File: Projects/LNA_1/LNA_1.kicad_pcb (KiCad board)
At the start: 2 copper layers, 59.7 x 36.6 mm, 31 parts, among them J1 SMA-J-P-H-ST-EM1, J2 SMA-J-P-H-ST-EM1, J3 Barrel_Jack_MountingPin, Q1 Q_NPN_BEC, U1 BFU790F

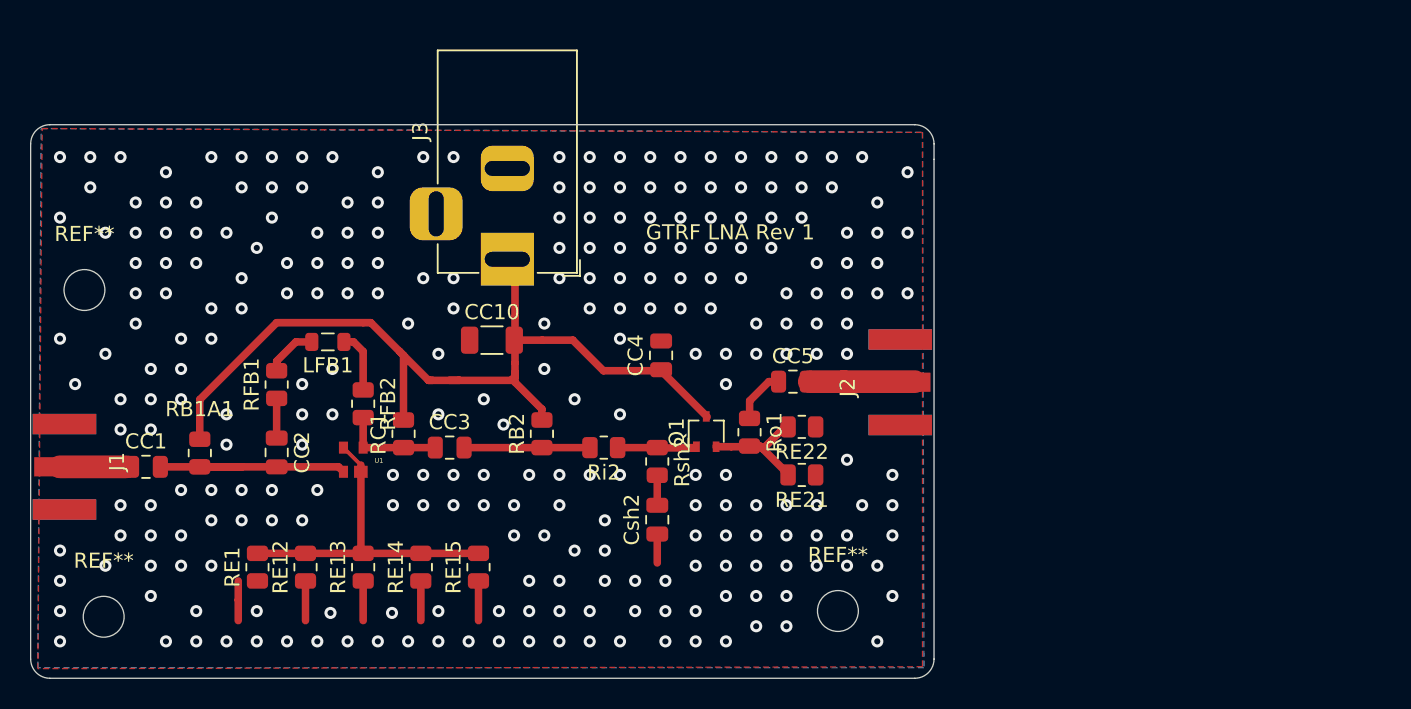
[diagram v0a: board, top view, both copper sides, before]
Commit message: This is the latest version with updated footprints etc
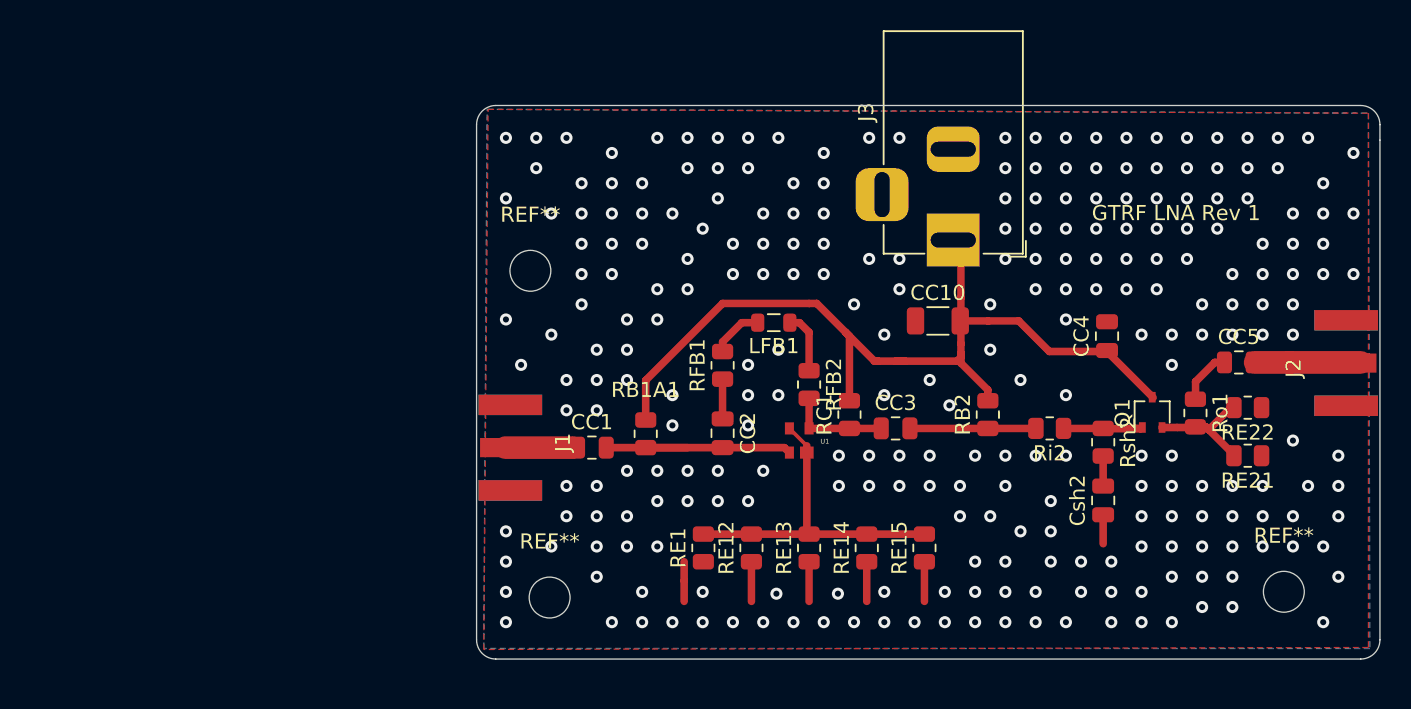
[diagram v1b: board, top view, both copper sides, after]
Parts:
- removed the REF** at (134.6, 78.1)
- removed the REF** at (86.1, 78.5)
- added REF**: MountingHole_2.7mm_M2.5, MountingHole:MountingHole_2.7mm_M2.5, F.Cu at (164.1, 76.8)
- added REF**: MountingHole_2.7mm_M2.5, MountingHole:MountingHole_2.7mm_M2.5, F.Cu at (115.6, 77.2)
- moved CC3 29.5 mm to (138.4, 66.0)
- moved J3 29.5 mm to (142.2, 53.6)
- moved RB2 29.5 mm to (144.5, 65.1)
- moved RE15 29.5 mm to (140.3, 73.9)
- moved CC1 29.5 mm to (118.4, 67.3)
- moved CC2 29.5 mm to (127.0, 66.4)
- moved CC4 29.5 mm to (152.4, 59.9)
- moved CC5 29.5 mm to (161.1, 61.7)
- moved J1 29.5 mm to (112.8, 67.3)
- moved J2 29.5 mm to (168.4, 61.7)
- moved LFB1 29.5 mm to (130.4, 59.1)
- moved RB1A1 29.5 mm to (121.9, 66.4)
- moved RC1 29.5 mm to (135.4, 65.1)
- moved RE1 29.5 mm to (125.7, 73.9)
- moved RE12 29.5 mm to (128.9, 73.9)
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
